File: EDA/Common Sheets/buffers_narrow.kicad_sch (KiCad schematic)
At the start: 18 parts, among them U4 74LVTH245, U5 74LVTH245, U6 74LVTH125, U7 74LVTH125, U8 SN74AHC1G125DBVR

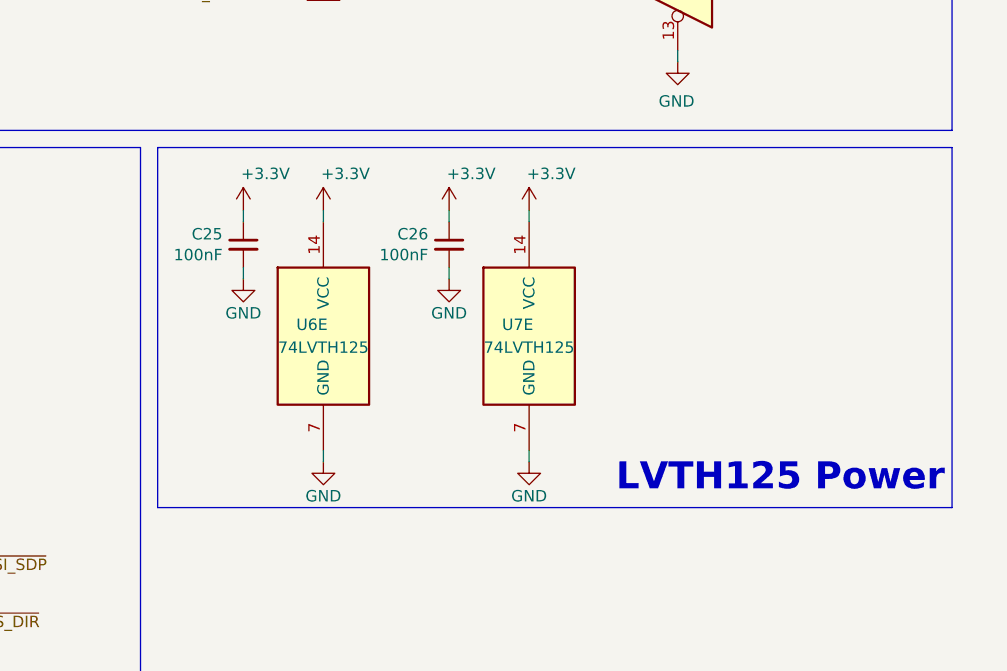
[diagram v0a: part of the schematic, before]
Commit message: Resuming work
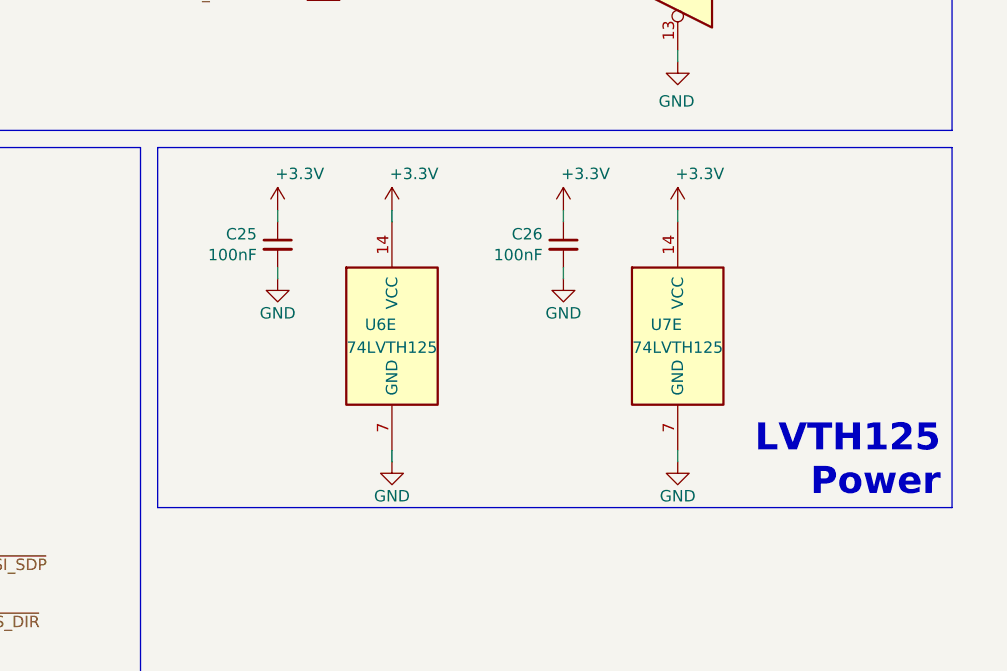
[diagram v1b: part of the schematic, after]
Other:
- moved on the sheet: C25, C26, U6E, U7E
